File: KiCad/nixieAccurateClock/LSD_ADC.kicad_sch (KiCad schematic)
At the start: 8 parts, among them U10 TXB0108DQSR, U11 TXB0108DQSR

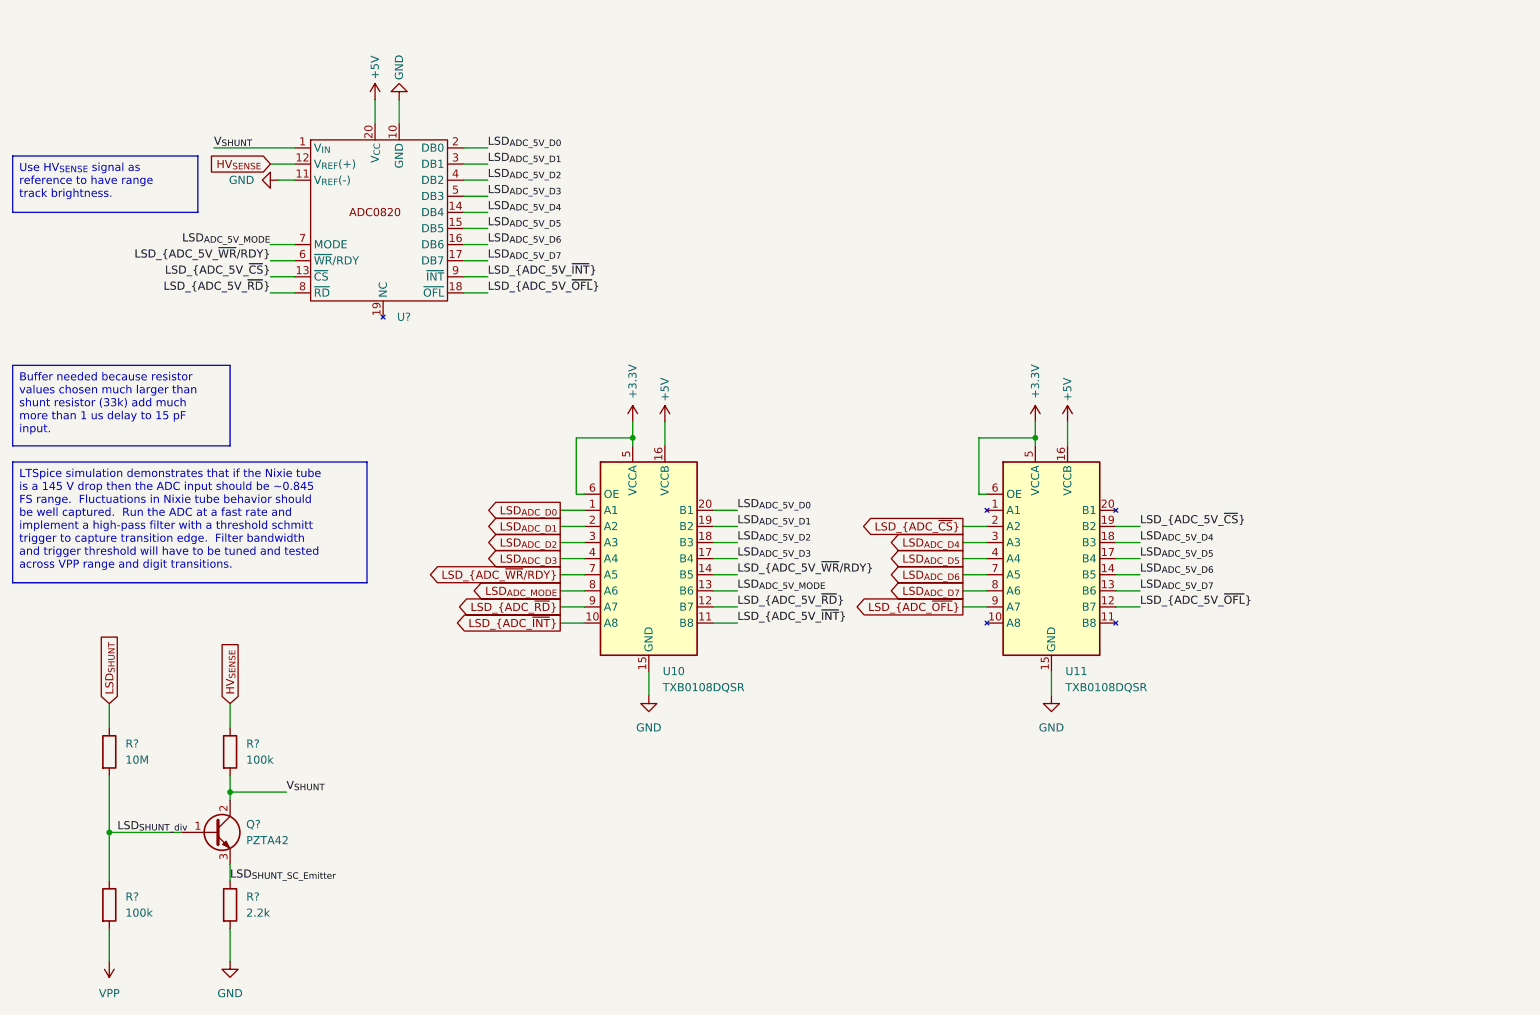
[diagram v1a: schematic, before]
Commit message: give pico iCE better mounting
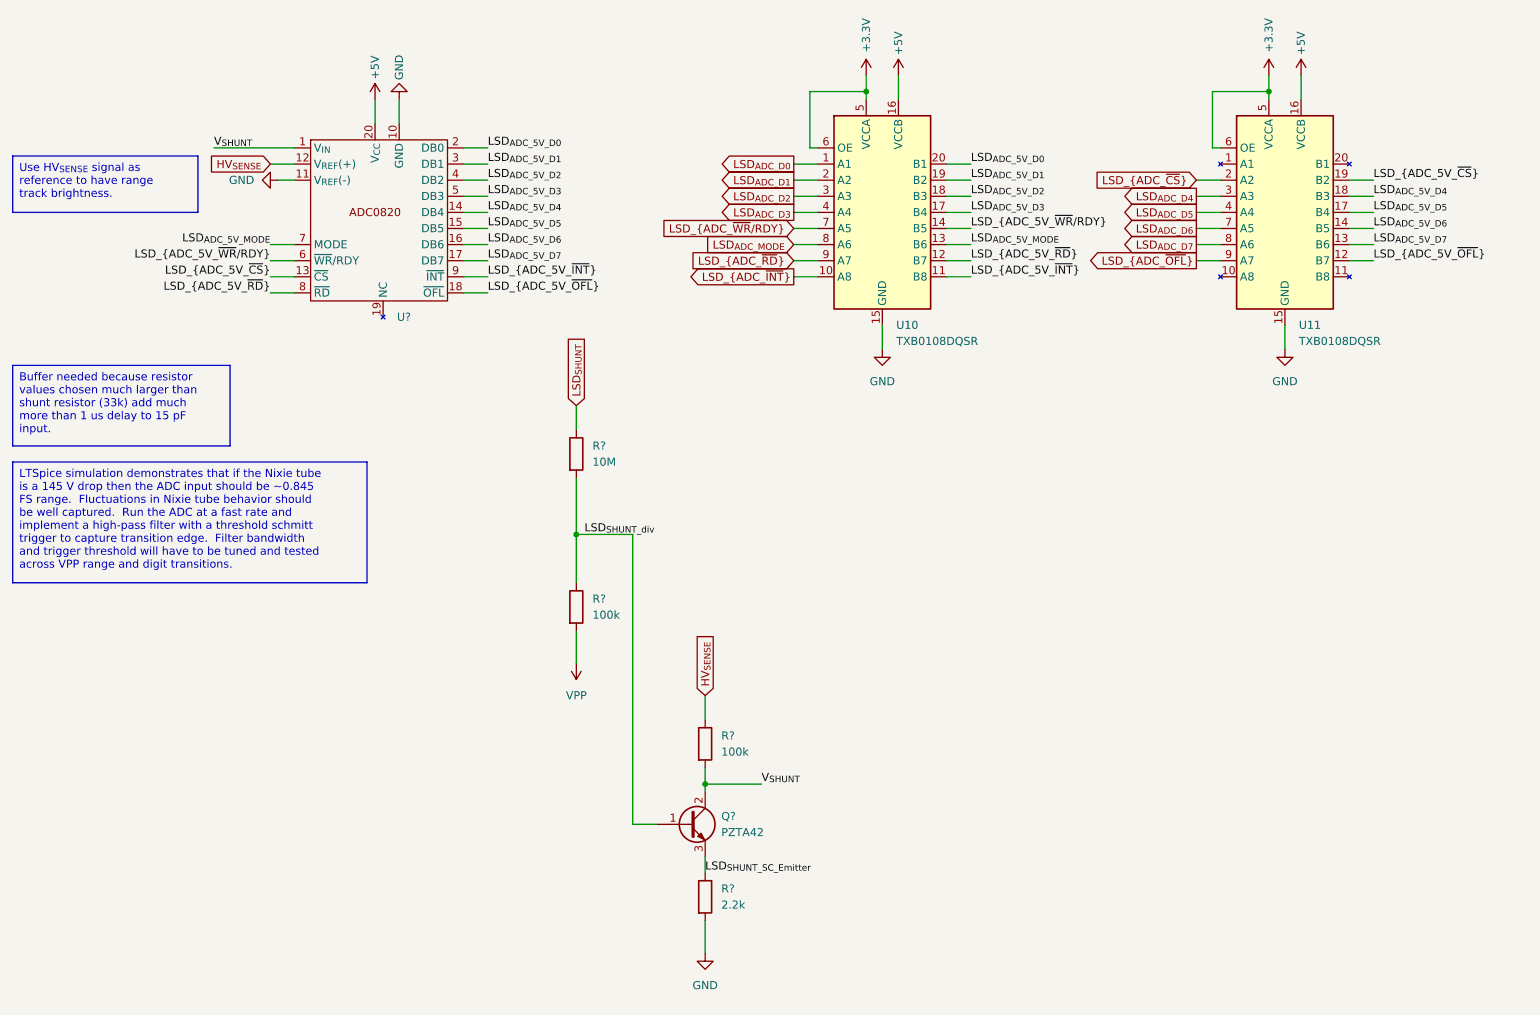
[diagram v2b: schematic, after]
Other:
- moved on the sheet: Q?, R?, U10, U11
